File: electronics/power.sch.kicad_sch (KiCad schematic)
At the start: 19 parts, among them Q2 MDD2301, U1 MCP73831-2-OT, U3 TLV74311, U4 TPS63000

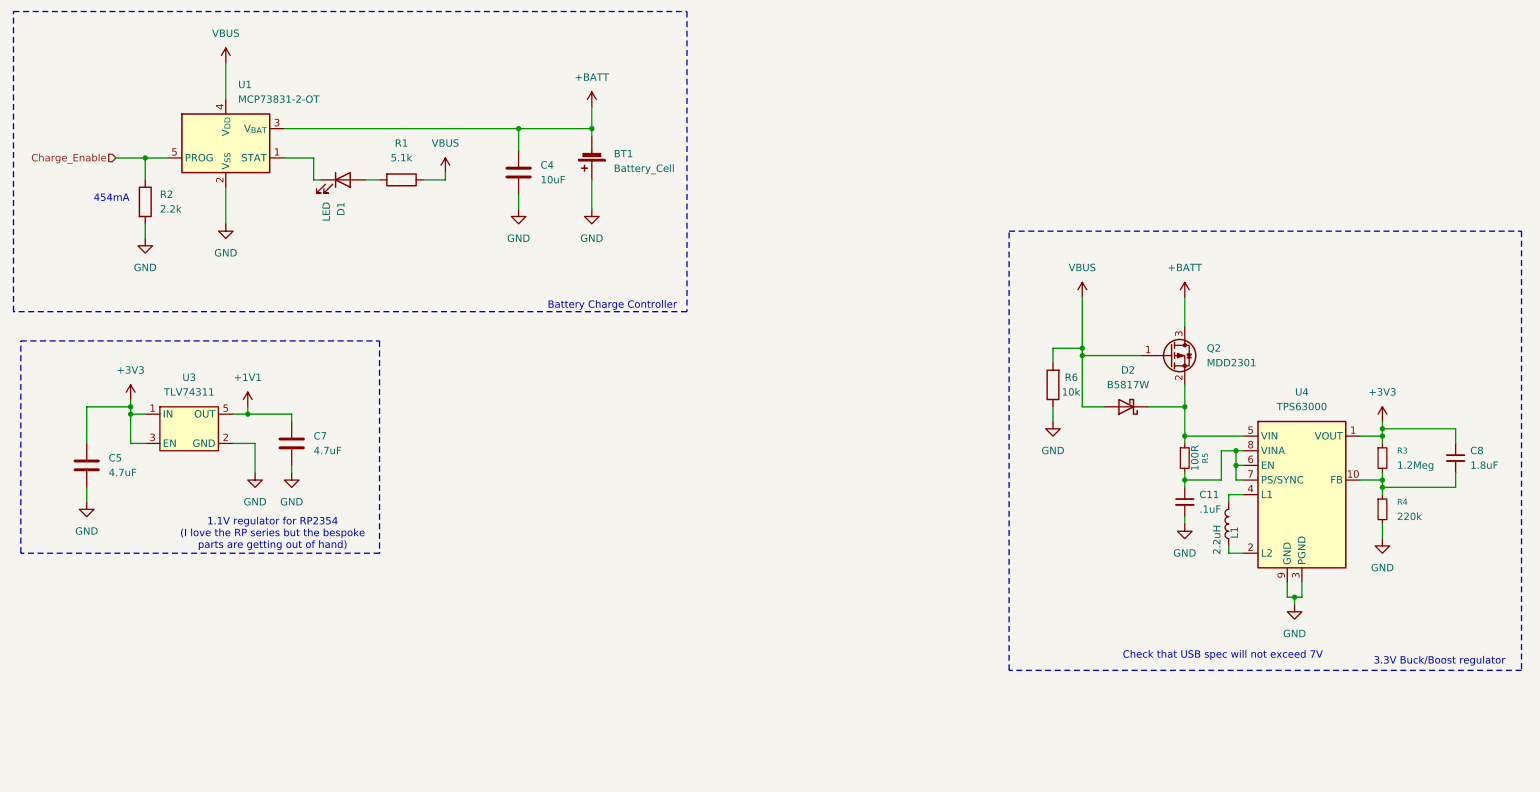
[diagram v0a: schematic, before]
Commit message: Microcontroller design
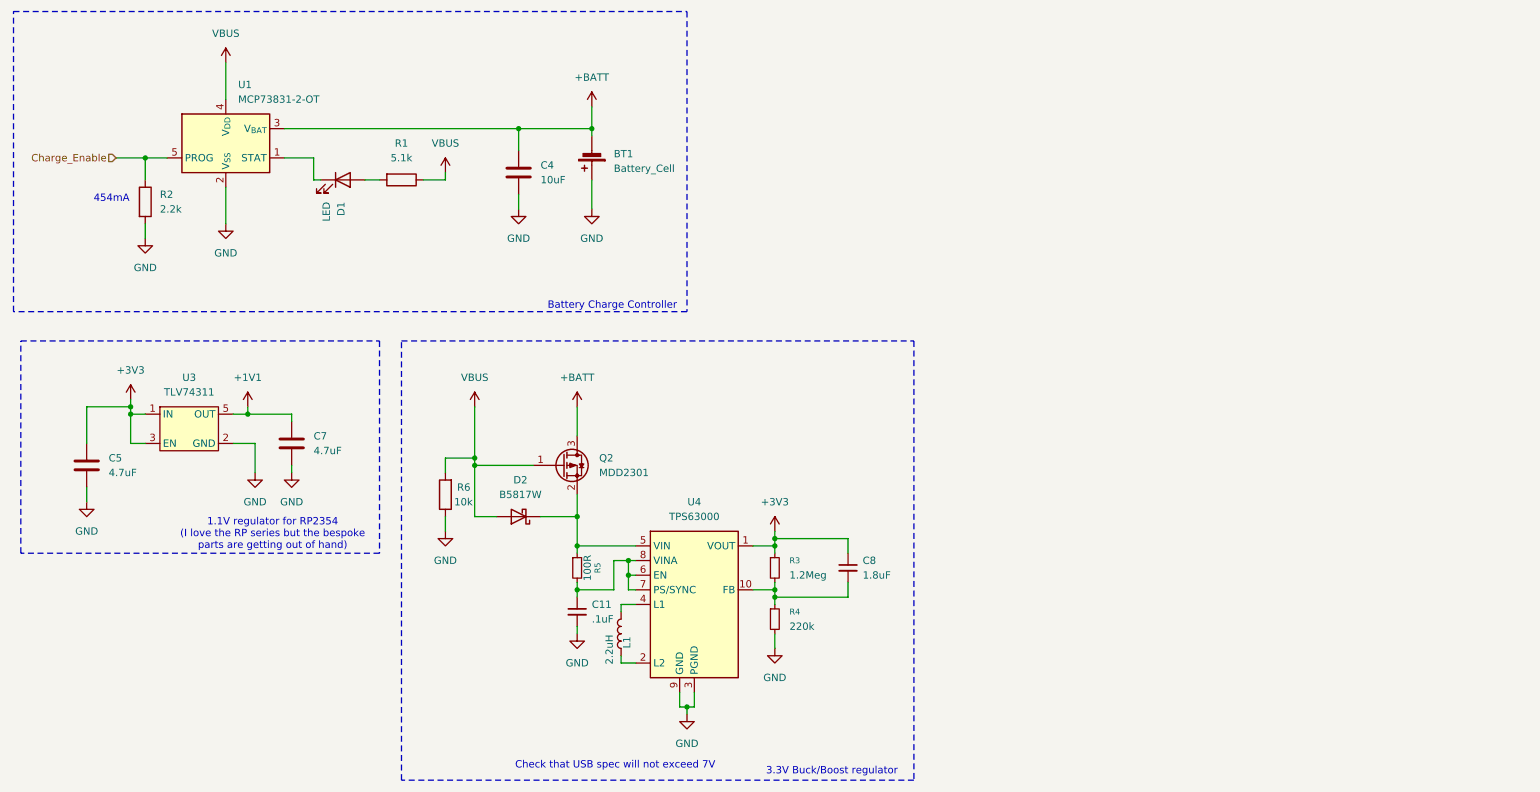
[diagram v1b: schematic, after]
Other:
- moved on the sheet: C11, C8, D2, L1, Q2, R3, R4, R5, R6, U4
